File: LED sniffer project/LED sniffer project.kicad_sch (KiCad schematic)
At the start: 12 parts, among them J1 Conn_01x02, J2 Conn_01x03, J3 Conn_01x03, J4 Conn_01x04, J5 Conn_01x04, SW1 Push_Button

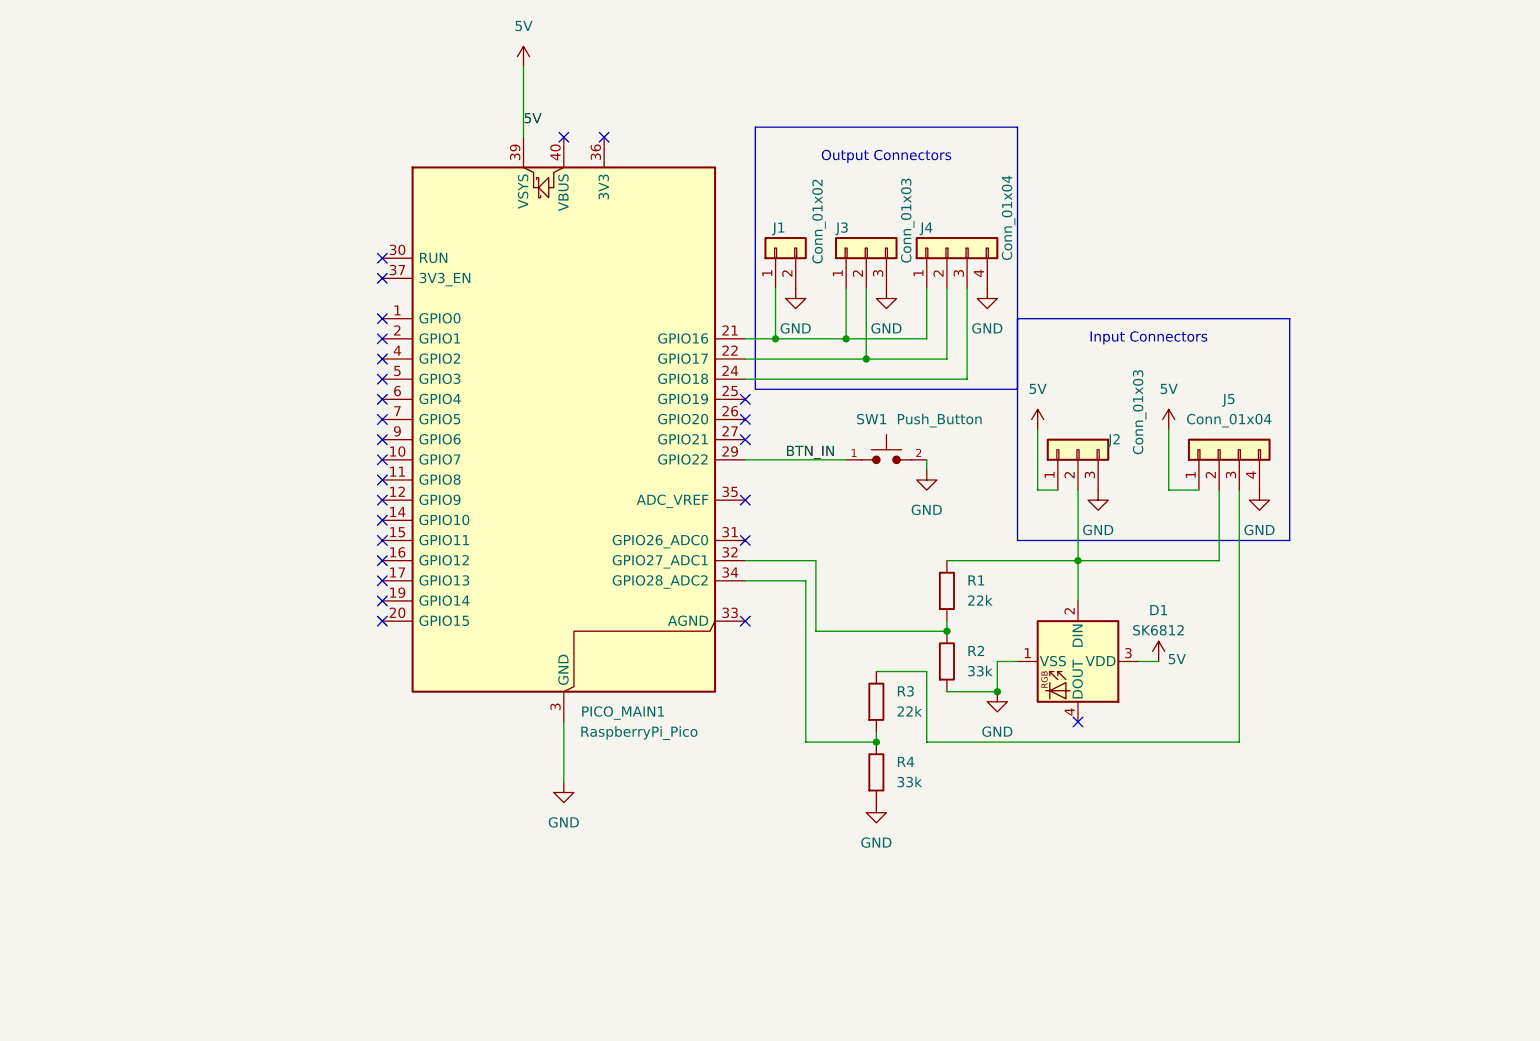
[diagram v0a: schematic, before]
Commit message: Possible submission
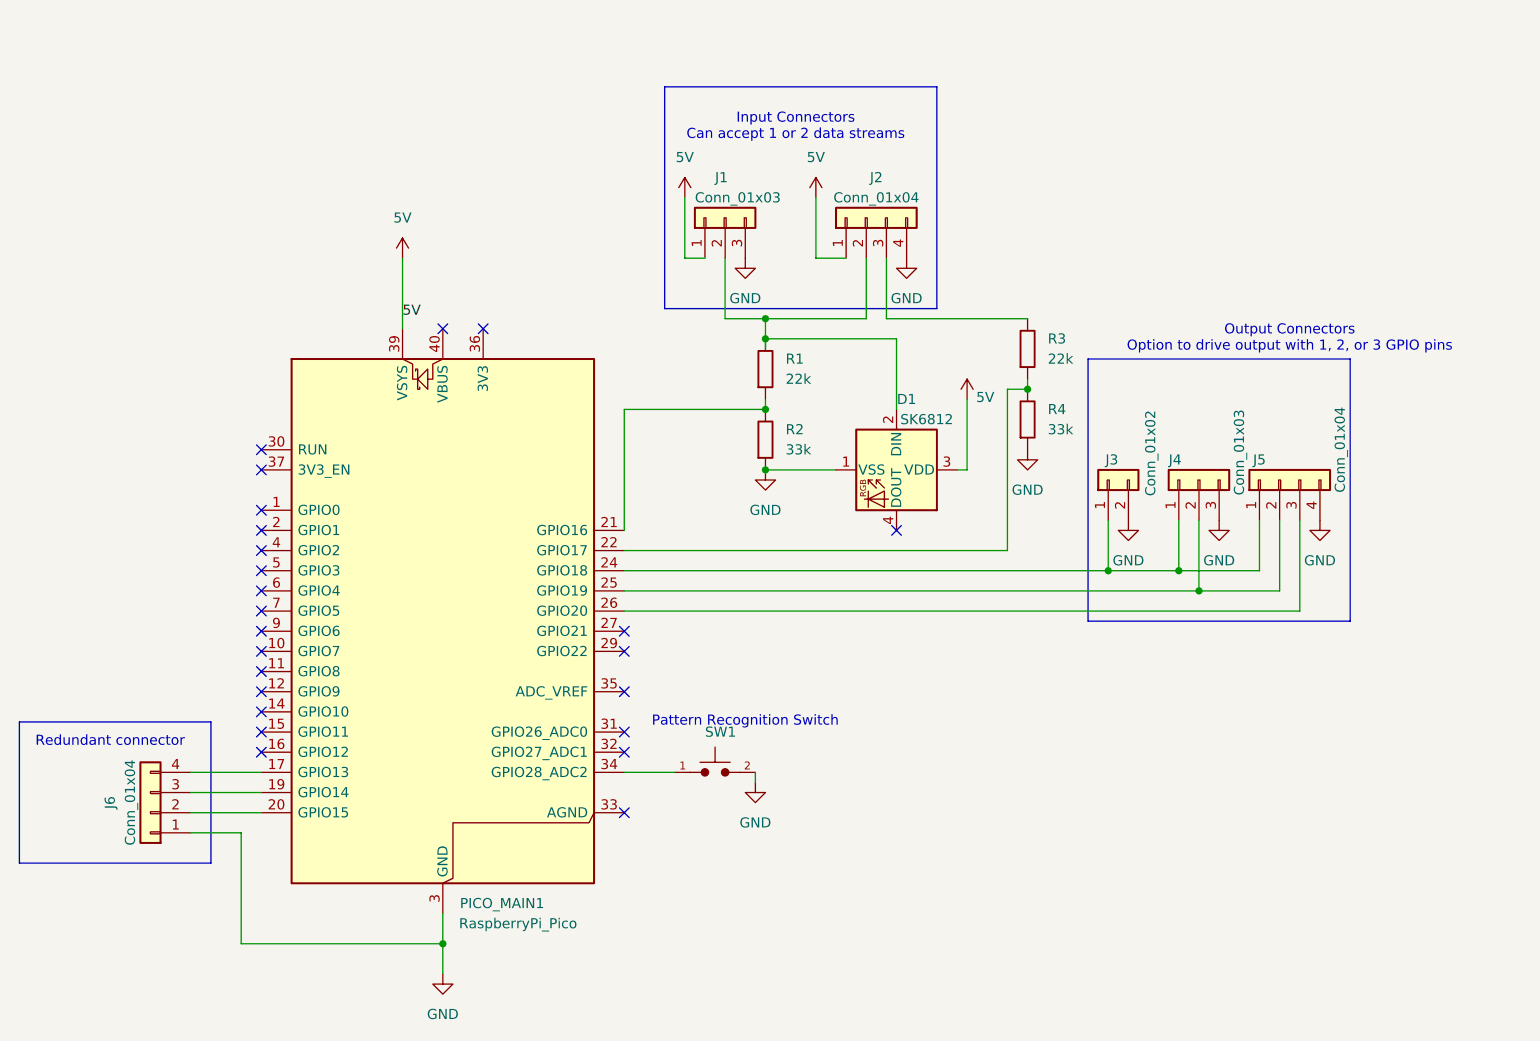
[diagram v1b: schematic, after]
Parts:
- added J6: Conn_01x04, Connector_PinHeader_2.54mm:PinHeader_1x04_P2.54mm_Vertical, symbol PCM_4ms_Connector:Conn_01x04
- renumbered J2 to J1, J5 to J2, J1 to J3, J3 to J4, J4 to J5
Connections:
- net GND: now also J6.1 (Pin_1)
- net at PICO_MAIN1.17 (GPIO13): now also J6.4 (Pin_4)
- net at PICO_MAIN1.19 (GPIO14): now also J6.3 (Pin_3)
- net at PICO_MAIN1.20 (GPIO15): now also J6.2 (Pin_2)
- net at J3.1 (Pin_1), J4.1 (Pin_1), J5.1 (Pin_1): now also PICO_MAIN1.24 (GPIO18); no longer PICO_MAIN1.21 (GPIO16)
- net at J4.2 (Pin_2), J5.2 (Pin_2): now also PICO_MAIN1.25 (GPIO19); no longer PICO_MAIN1.22 (GPIO17)
- net at J5.3 (Pin_3): now also PICO_MAIN1.26 (GPIO20); no longer PICO_MAIN1.24 (GPIO18)
- net at R1.1, R2.2: now also PICO_MAIN1.21 (GPIO16); no longer PICO_MAIN1.32 (GPIO27_ADC1)
- net at R3.1, R4.2: now also PICO_MAIN1.22 (GPIO17); no longer PICO_MAIN1.34 (GPIO28_ADC2)
- net BTN_IN: no longer names the net of PICO_MAIN1.29 (GPIO22)
- net BTN_IN: no longer SW1.1
- new net: PICO_MAIN1.34 (GPIO28_ADC2), SW1.1
- no-connect marks 27 -> 24
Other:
- note added: "Input Connectors Can accept 1 or 2 data streams"
- note added: "Output Connectors Option to drive output with 1, 2, or 3 GPIO pins"
- note added: "Pattern Recognition Switch"
- note added: "Redundant connector"
- note removed: "Input Connectors"
- note removed: "Output Connectors"
- moved on the sheet: D1, J1, J2, J3, J4, J5, PICO_MAIN1, R1, R2, R3, R4, SW1
